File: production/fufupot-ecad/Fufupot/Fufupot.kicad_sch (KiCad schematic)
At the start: 56 parts, among them IC1 FOD3150, J1 Conn_01x04, J1 USB_B, J10 Conn_01x03, J11 Conn_01x03, J12 Conn_01x02, J3 Conn_01x03, J4 Conn_01x02, J5 Conn_01x02, J6 Conn_01x02, J7 Conn_01x02, J8 Conn_01x04, J9 Conn_01x02, SW1 SW_Push, U1 STGP8NC60KD, U2 FT232RL, U2 LM5165DRC, U3 USBLC6-2SC6, U4 ATMEGA328P-PN

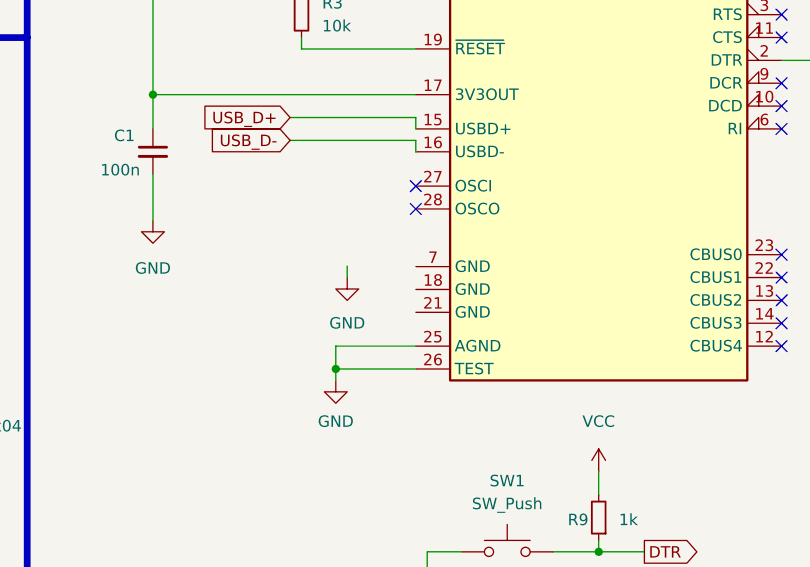
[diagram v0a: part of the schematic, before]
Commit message: Fixed GND issues
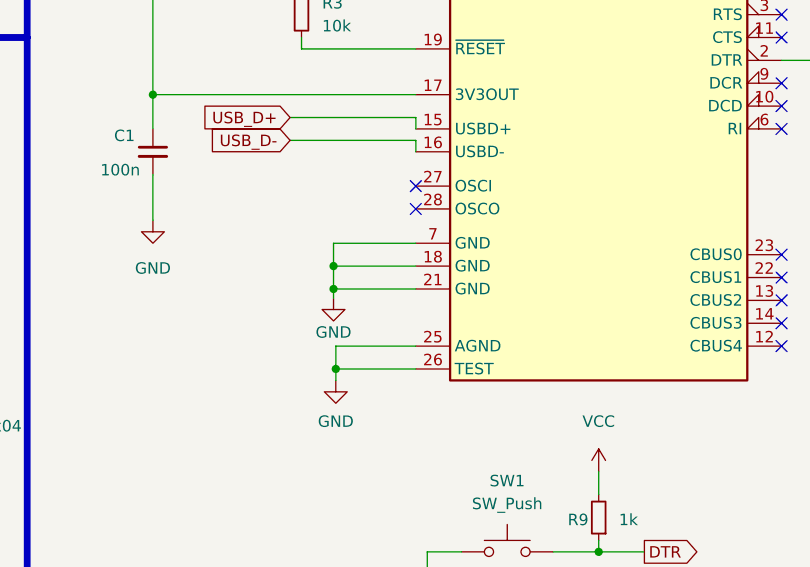
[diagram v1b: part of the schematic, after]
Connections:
- net GND: now also U2.18 (GND), U2.21 (GND), U2.7 (GND)
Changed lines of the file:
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@@
   (junction (at 304.8 210.82) (diameter 0) (color 0 0 0 0)
   )
+  (junction (at 175.006 238.76) (diameter 0) (color 0 0 0 0)
+  )
   (junction (at 320.04 100.33) (diameter 0) (color 0 0 0 0)
   )
@@
   (junction (at 322.58 113.03) (diameter 0) (color 0 0 0 0)
   )
+  (junction (at 175.006 236.22) (diameter 0) (color 0 0 0 0)
+  )
   (junction (at 370.84 57.15) (diameter 0) (color 0 0 0 0)
   )
@@
   (junction (at 49.53 48.26) (diameter 0) (color 0 0 0 0)
   )
-  (no_connect (at 184.15 229.87))
   (no_connect (at 128.27 43.18))
   (no_connect (at 224.79 215.9))
@@
   (no_connect (at 224.79 240.03))
   (no_connect (at 128.27 45.72))
+  (no_connect (at 184.15 229.87))
   (no_connect (at 184.15 227.33))
   (no_connect (at 224.79 234.95))
@@
     (stroke (width 0) (type default))
   )
-  (wire (pts (xy 176.53 236.22) (xy 176.53 237.49))
-    (stroke (width 0) (type default))
-  )
   (wire (pts (xy 288.29 210.82) (xy 304.8 210.82))
     (stroke (width 0) (type default))
@@
     (stroke (width 0) (type default))
   )
+  (wire (pts (xy 184.15 236.22) (xy 175.006 236.22))
+    (stroke (width 0) (type default))
+  )
   (wire (pts (xy 341.63 57.15) (xy 341.63 62.23))
     (stroke (width 0) (type default))
@@
   )
   (wire (pts (xy 360.68 224.79) (xy 367.03 224.79))
+    (stroke (width 0) (type default))
+  )
+  (wire (pts (xy 175.006 233.68) (xy 175.006 236.22))
     (stroke (width 0) (type default))
   )
@@
     (stroke (width 0) (type default))
   )
+  (wire (pts (xy 175.006 238.76) (xy 175.006 239.776))
+    (stroke (width 0) (type default))
+  )
   (polyline (pts (xy 231.14 12.7) (xy 231.14 74.93))
     (stroke (width 0.75) (type default))
@@
     (stroke (width 0) (type default))
   )
+  (wire (pts (xy 175.006 236.22) (xy 175.006 238.76))
+    (stroke (width 0) (type default))
+  )
   (wire (pts (xy 154.94 217.17) (xy 184.15 217.17))
     (stroke (width 0) (type default))
@@
     (stroke (width 0) (type default))
   )
+  (wire (pts (xy 184.15 233.68) (xy 175.006 233.68))
+    (stroke (width 0) (type default))
+  )
   (wire (pts (xy 370.84 85.09) (xy 370.84 93.98))
     (stroke (width 0) (type default))
@@
   (polyline (pts (xy 76.2 144.78) (xy 76.2 210.82))
     (stroke (width 0.75) (type default))
+  )
+  (wire (pts (xy 184.15 238.76) (xy 175.006 238.76))
+    (stroke (width 0) (type default))
   )
   (wire (pts (xy 370.84 34.29) (xy 370.84 36.83))
@@
     )
   )
-  (symbol (lib_id "power:GND") (at 176.53 237.49 0) (unit 1)
-    (in_bom yes) (on_board yes) (dnp no) (fields_autoplaced)
-    (property "Reference" "#PWR047" (at 176.53 243.84 0)
-      (effects (font (size 1.27 1.27)) hide)
-    )
-    (property "Value" "GND" (at 176.53 242.57 0)
-      (effects (font (size 1.27 1.27)))
-    )
-    (property "Footprint" "" (at 176.53 237.49 0)
-      (effects (font (size 1.27 1.27)) hide)
-    )
-    (property "Datasheet" "" (at 176.53 237.49 0)
-      (effects (font (size 1.27 1.27)) hide)
-    )
-    (pin "1")
-    (instances
-      (project "Fufupot"
-        (path "/e8bc21b1-eda8-45a8-be25-55b90339183f"
-          (reference "#PWR047") (unit 1)
-        )
-      )
-    )
-  )
   (symbol (lib_id "Device:R") (at 153.67 54.61 0) (unit 1)
     (in_bom yes) (on_board yes) (dnp no)
@@
         )
       )
+    )
+  )
+  (symbol (lib_id "power:GND") (at 175.006 239.776 0) (unit 1)
+    (in_bom yes) (on_board yes) (dnp no)
+    (property "Reference" "#PWR047" (at 175.006 246.126 0)
+      (effects (font (size 1.27 1.27)) hide)
+    )
+    (property "Value" "GND" (at 175.006 243.586 0)
+      (effects (font (size 1.27 1.27)))
+    )
+    (property "Footprint" "" (at 175.006 239.776 0)
+      (effects (font (size 1.27 1.27)) hide)
+    )
+    (property "Datasheet" "" (at 175.006 239.776 0)
+      (effects (font (size 1.27 1.27)) hide)
+    )
+    (pin "1")
+    (instances
+      (project "Fufupot"
+        (path "/e8bc21b1-eda8-45a8-be25-55b90339183f"
+          (reference "#PWR047") (unit 1)
+        )
+      )
